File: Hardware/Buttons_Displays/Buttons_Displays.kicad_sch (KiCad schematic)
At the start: 12 parts, among them J1 Conn_01x10, J2 Conn_01x10, J3 Conn_01x10, J4 Conn_01x10, J5 Conn_01x10, J6 Conn_01x10, J7 Conn_01x10, J8 Conn_01x10, J9 Conn_01x03, U1 STM32H523RETx

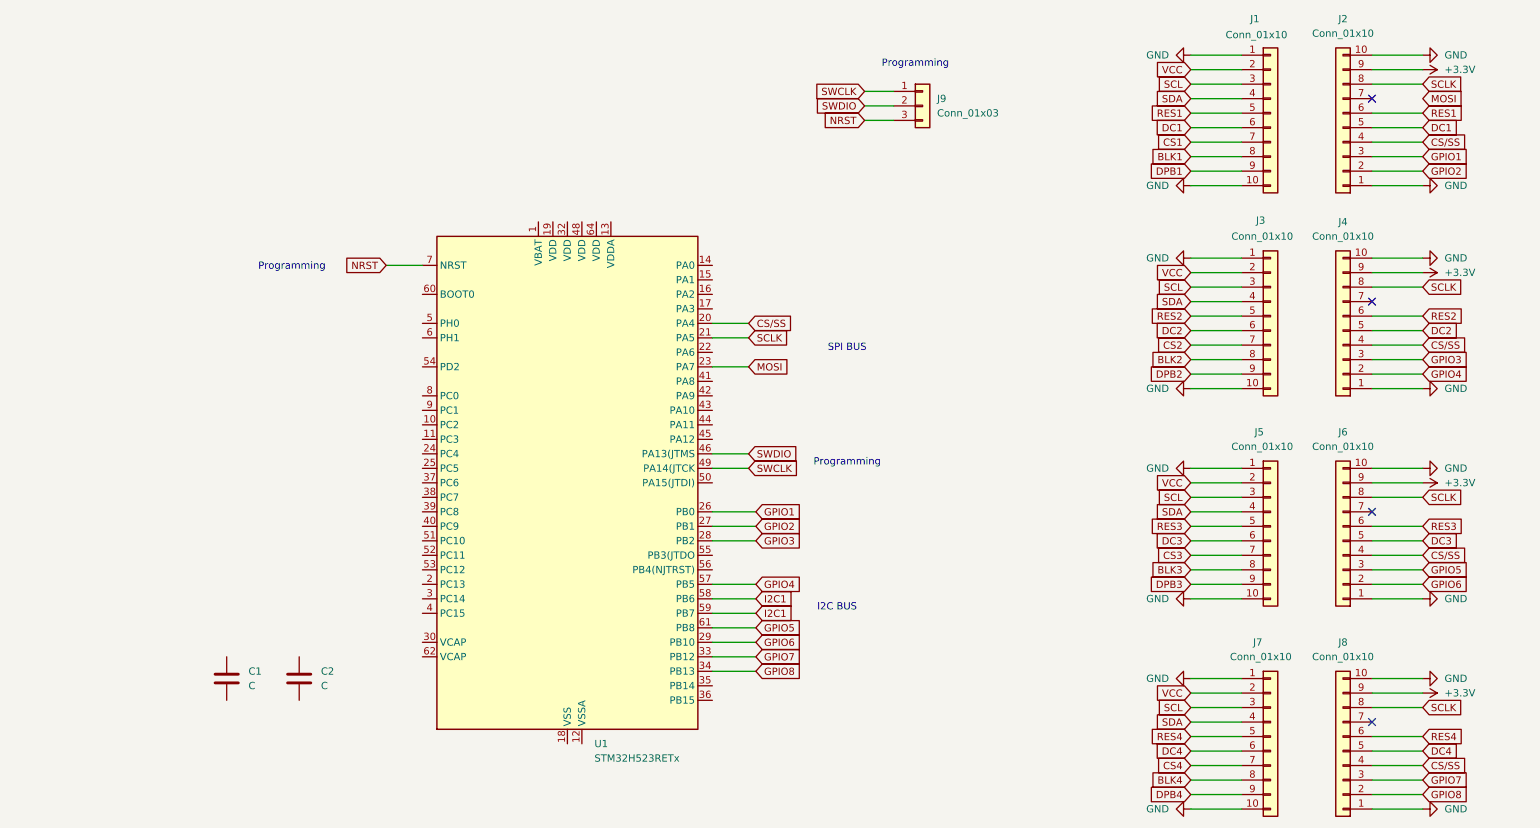
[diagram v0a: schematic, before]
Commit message: mierenneukerij
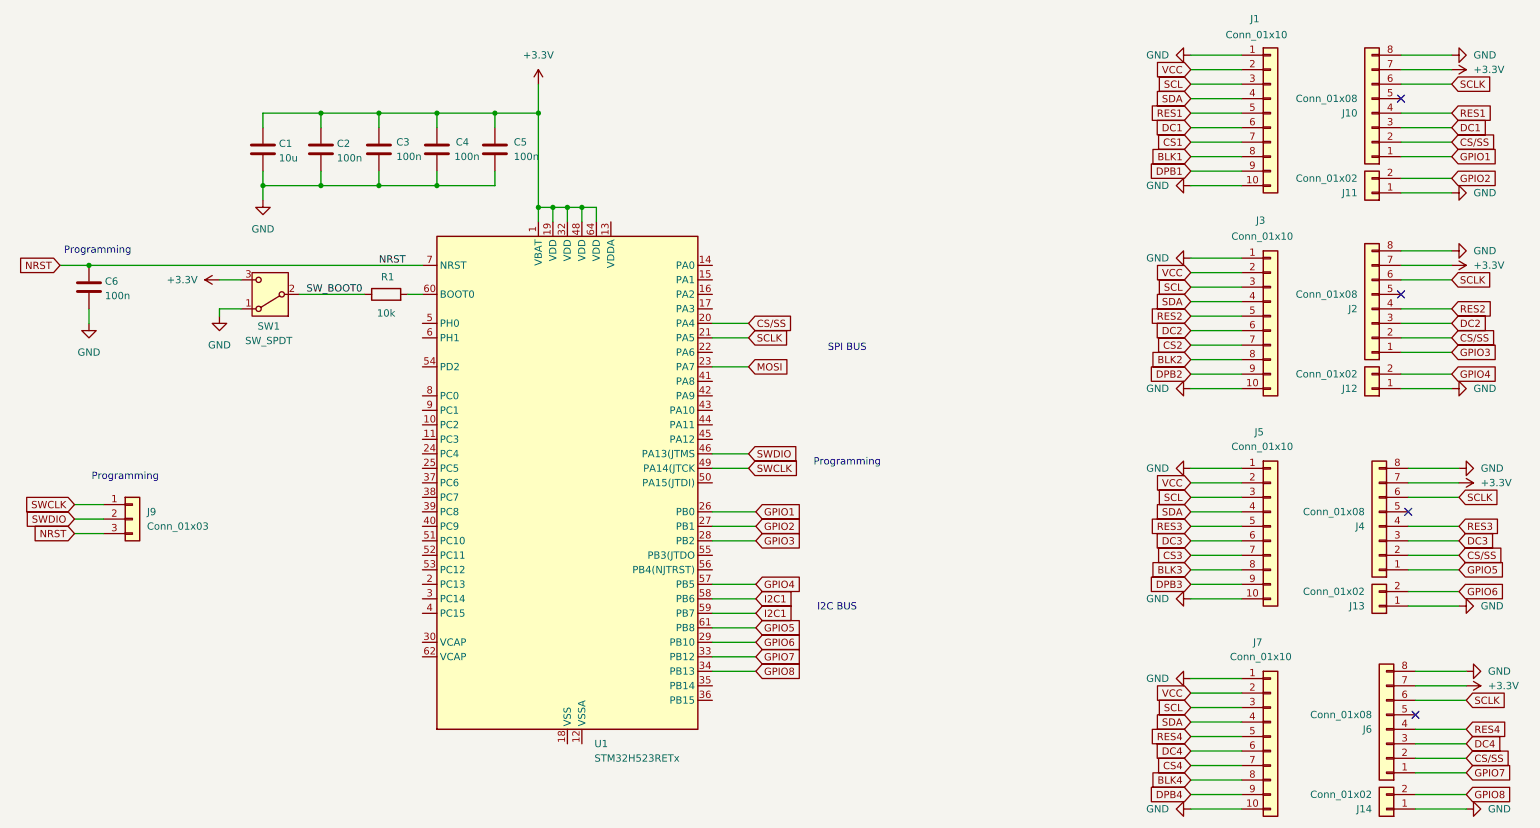
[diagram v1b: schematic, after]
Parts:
- removed J2, J4, J6, J8: Conn_01x10, symbol Connector_Generic:Conn_01x10
- added C3, C4, C5, C6: 100n, Capacitor_SMD:C_1206_3216Metric_Pad1.33x1.80mm_HandSolder, symbol Device:C
- added J10, J2, J4, J6: Conn_01x08, symbol Connector_Generic:Conn_01x08
- added J11, J12, J13, J14: Conn_01x02, symbol Connector_Generic:Conn_01x02
- added R1: 10k, symbol Device:R
- added SW1: SW_SPDT, symbol Switch:SW_SPDT
- C1: value C -> 10u
- C2: value C -> 100n
- J1: footprint (none) -> ConnectorPT:1778609
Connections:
- net +3.3V: now also C1.1, C2.1, U1.1 (VBAT), U1.19 (VDD), U1.32 (VDD), U1.48 (VDD), U1.64 (VDD), C3.1, C4.1, C5.1, J10.7 (Pin_7), J2.7 (Pin_7), J4.7 (Pin_7), J6.7 (Pin_7), SW1.3 (C)
- net CS/SS: now also J10.2 (Pin_2), J2.2 (Pin_2), J4.2 (Pin_2), J6.2 (Pin_2)
- net DC1: now also J10.3 (Pin_3)
- net DC2: now also J2.3 (Pin_3)
- net DC3: now also J4.3 (Pin_3)
- net DC4: now also J6.3 (Pin_3)
- net GND: now also C1.2, C2.2, C3.2, C4.2, C5.2, C6.2, J10.8 (Pin_8), J11.1 (Pin_1), J12.1 (Pin_1), J13.1 (Pin_1), J14.1 (Pin_1), J2.8 (Pin_8), J4.8 (Pin_8), J6.8 (Pin_8), SW1.1 (A)
- net GPIO1: now also J10.1 (Pin_1)
- net GPIO2: now also J11.2 (Pin_2)
- net GPIO3: now also J2.1 (Pin_1)
- net GPIO4: now also J12.2 (Pin_2)
- net GPIO5: now also J4.1 (Pin_1)
- net GPIO6: now also J13.2 (Pin_2)
- net GPIO7: now also J6.1 (Pin_1)
- net GPIO8: now also J14.2 (Pin_2)
- net NRST: now also C6.1
- net RES1: now also J10.4 (Pin_4)
- net RES2: now also J2.4 (Pin_4)
- net RES3: now also J4.4 (Pin_4)
- net RES4: now also J6.4 (Pin_4)
- net SCLK: now also J10.6 (Pin_6), J2.6 (Pin_6), J4.6 (Pin_6), J6.6 (Pin_6)
- net at U1.60 (BOOT0): now also R1.2
- new net SW_BOOT0: R1.1, SW1.2 (B)
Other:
- moved on the sheet: C1, C2, J9
